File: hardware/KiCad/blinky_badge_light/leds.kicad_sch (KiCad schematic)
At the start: 48 parts

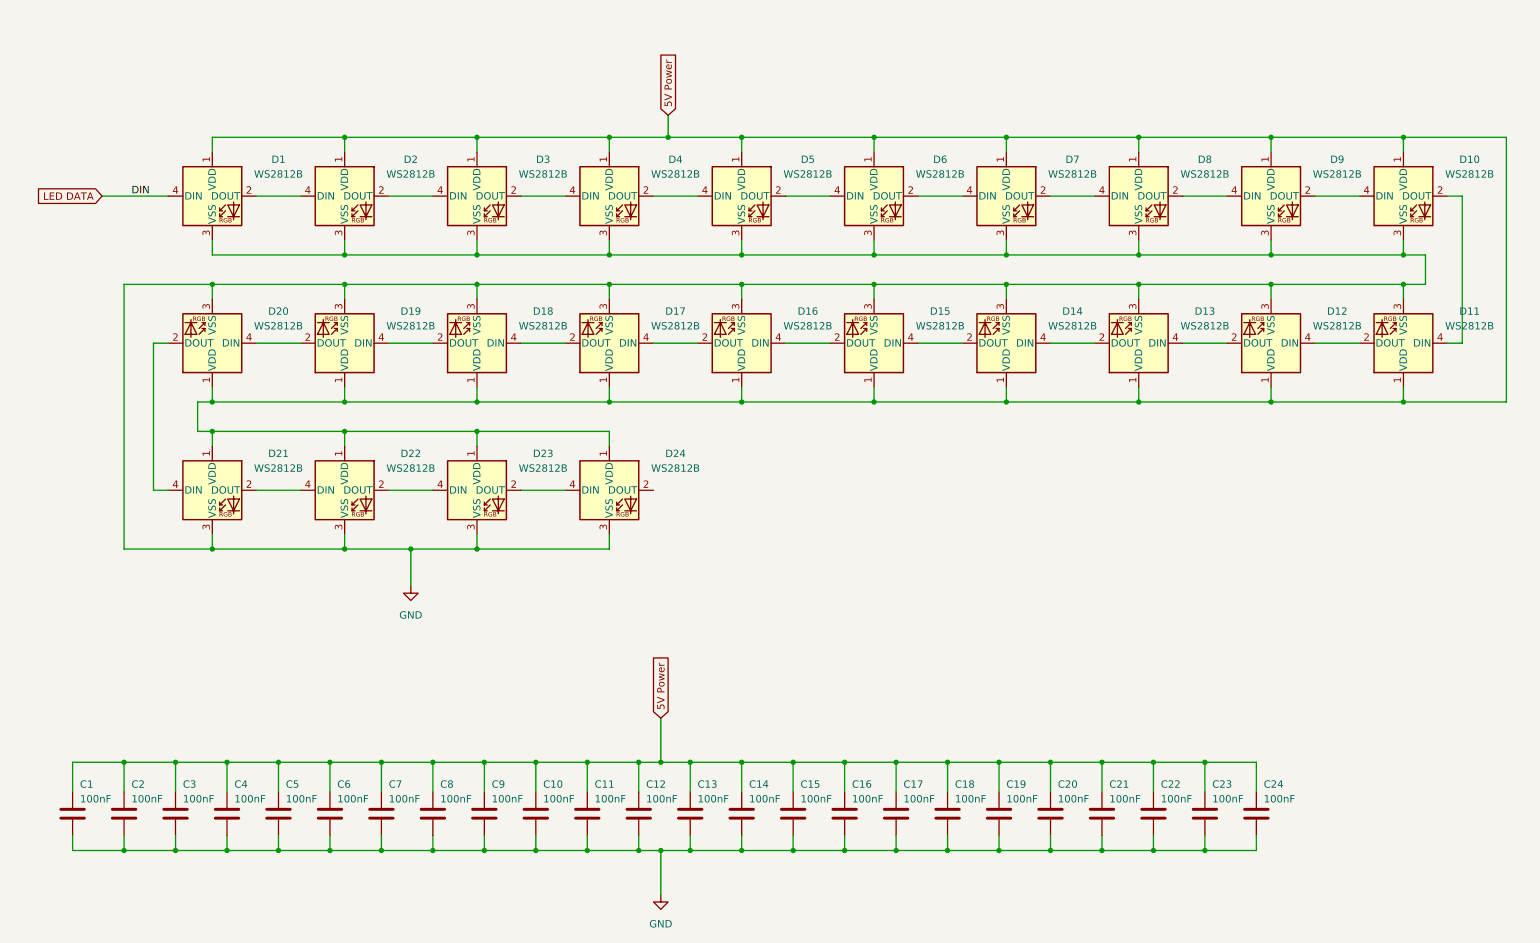
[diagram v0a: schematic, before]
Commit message: updates to hardware schematic
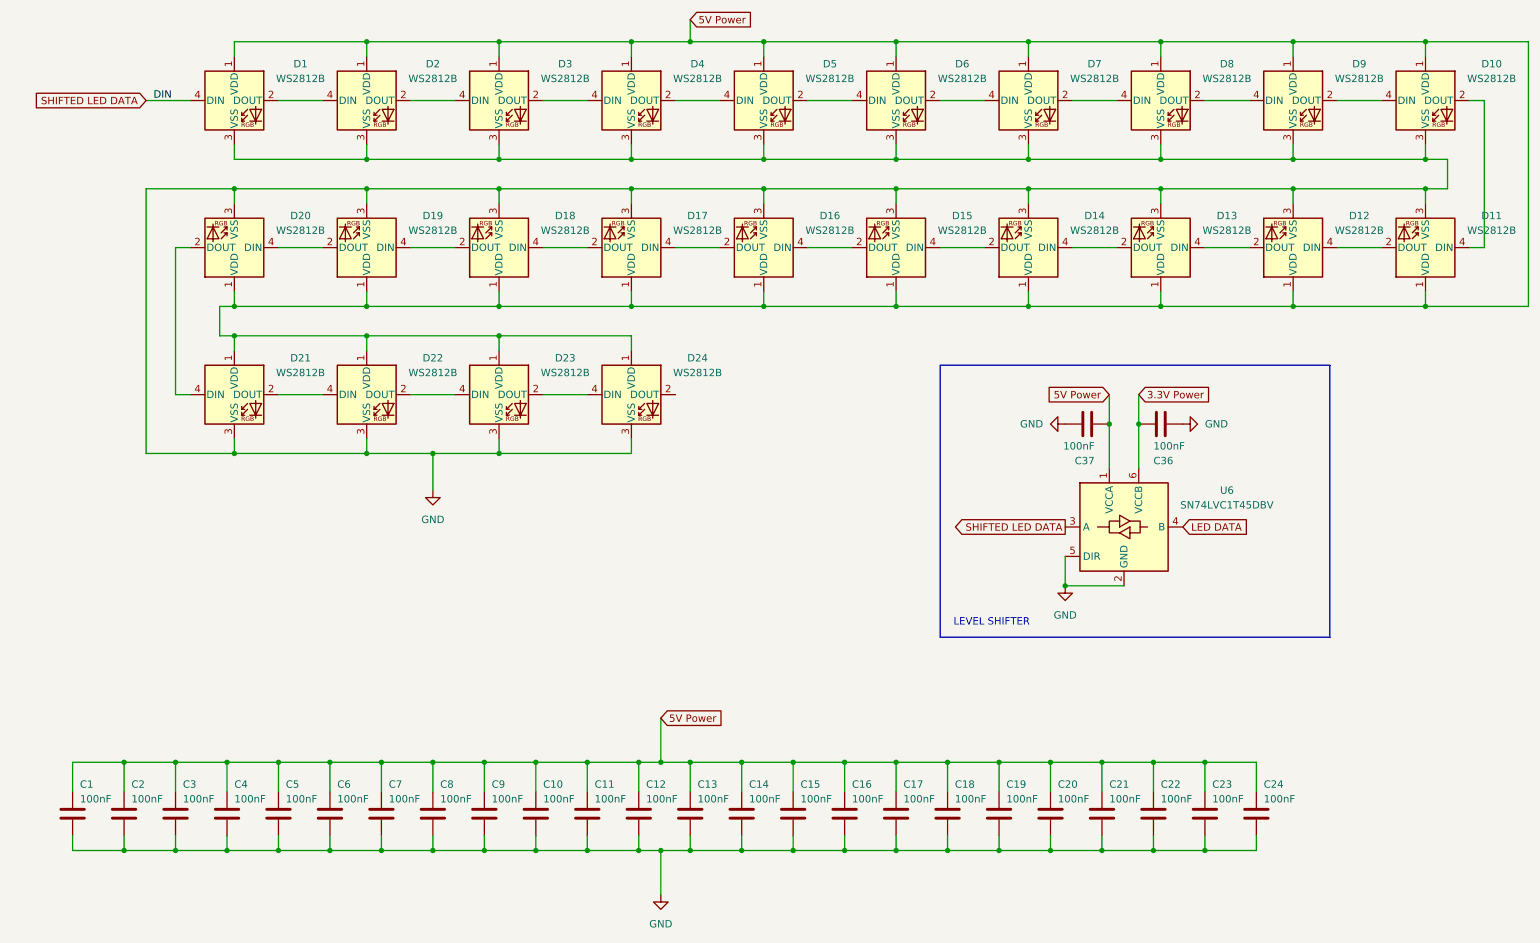
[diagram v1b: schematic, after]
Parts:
- added C36, C37: 100nF, Capacitor_SMD:C_0402_1005Metric, symbol Device:C
- added U6: SN74LVC1T45DBV, Package_TO_SOT_SMD:SOT-23-6, symbol Logic_LevelTranslator:SN74LVC1T45DBV
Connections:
- net 5V Power: now also C37.2, U6.1 (VCCA)
- net GND: now also C36.1, C37.1, U6.2 (GND), U6.5 (DIR)
- net LED DATA: now also U6.4 (B); no longer D1.4 (DIN)
- new net 3.3V Power: C36.2, U6.6 (VCCB)
- new net SHIFTED LED DATA: D1.4 (DIN), U6.3 (A)
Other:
- note added: "LEVEL SHIFTER"
- moved on the sheet: D1, D10, D11, D12, D13, D14, D15, D16, D17, D18, D19, D2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

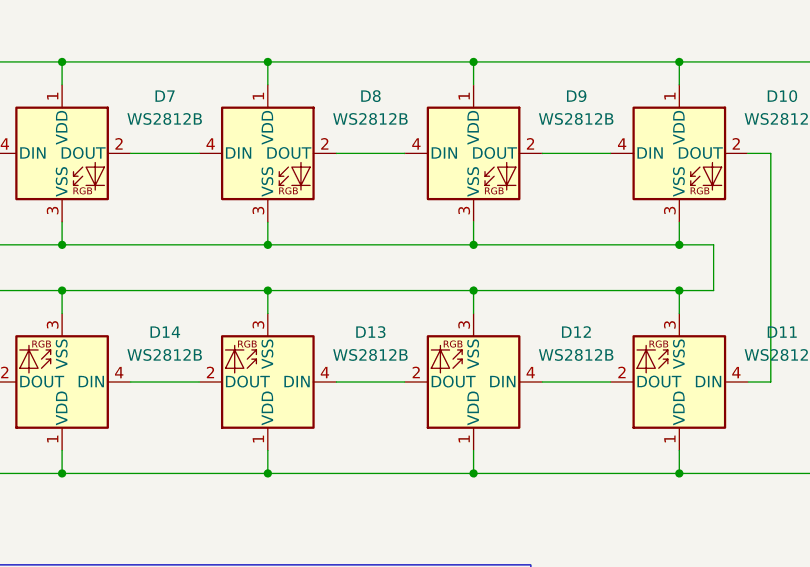
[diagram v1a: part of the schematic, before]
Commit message: placing items on the board
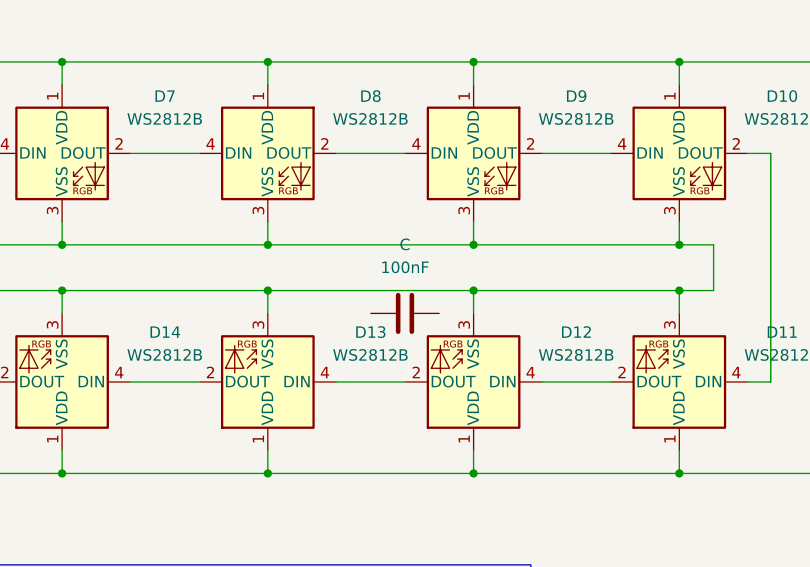
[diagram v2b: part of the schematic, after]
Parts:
- added C: 100nF, Capacitor_SMD:C_0402_1005Metric, symbol Device:C
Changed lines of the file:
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@@
+	)
+	(symbol
+		(lib_id "Device:C")
+		(at 228.6 49.53 90)
+		(unit 1)
+		(exclude_from_sim no)
+		(in_bom yes)
+		(on_board yes)
+		(dnp no)
+		(fields_autoplaced yes)
+		(property "Reference" "C"
+			(at 228.6 41.91 90)
+			(effects
+				(font
+					(size 1.27 1.27)
+				)
+			)
+		)
+		(property "Value" "100nF"
+			(at 228.6 44.45 90)
+			(effects
+				(font
+					(size 1.27 1.27)
+				)
+			)
+		)
+		(property "Footprint" "Capacitor_SMD:C_0402_1005Metric"
+			(at 232.41 48.5648 0)
+			(effects
+				(font
+					(size 1.27 1.27)
+				)
+				(hide yes)
+			)
+		)
+		(property "Datasheet" "https://www.lcsc.com/datasheet/lcsc_datasheet_2304140030_Samsung-Electro-Mechanics-CL05B104KO5NNNC_C1525.pdf"
+			(at 228.6 49.53 0)
+			(effects
+				(font
+					(size 1.27 1.27)
+				)
+				(hide yes)
+			)
+		)
+		(property "Description" "Unpolarized capacitor"
+			(at 228.6 49.53 0)
+			(effects
+				(font
+					(size 1.27 1.27)
+				)
+				(hide yes)
+			)
+		)
+		(property "JLCPCB Part #" "C1525"
+			(at 228.6 49.53 0)
+			(effects
+				(font
+					(size 1.27 1.27)
+				)
+				(hide yes)
+			)
+		)
+		(pin "1"
+		)
+		(pin "2"
+		)
+		(instances
+			(project "blinky_badge_light"
+				(path "/f33039b1-b38b-4cb6-baf0-07a137773378/a31a264e-f1c4-410a-a175-a81c007586a2"
+					(reference "C29")
+					(unit 1)
+				)
+			)
+		)
 	)
 	(symbol
